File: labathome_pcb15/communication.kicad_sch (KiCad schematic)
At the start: 19 parts, among them M1 W5500_mini, SW2 ON RS TERM, SW3 ON CAN TERM, U1 MAX3485, U15 NRF24L01, U6 RFM95W-868S2, U7 SN65HVD230, X3 SIM7080G

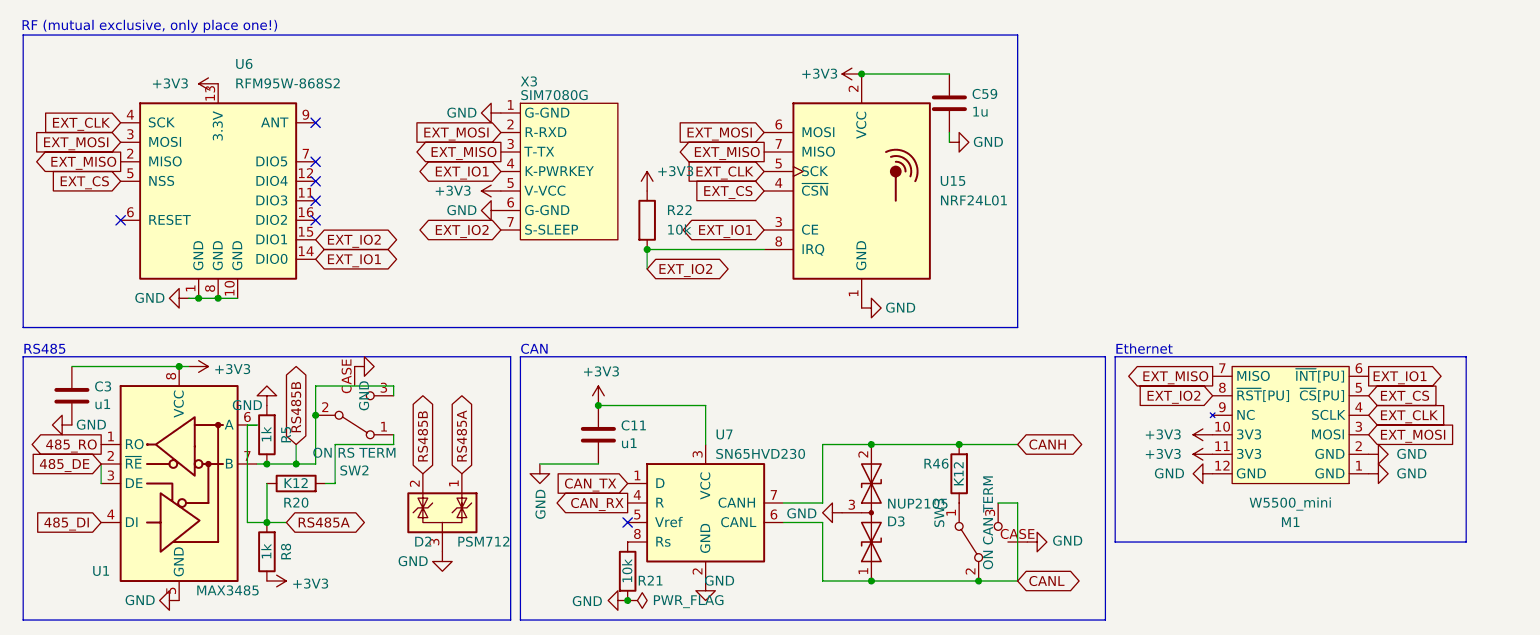
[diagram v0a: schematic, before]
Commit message: Minimal changes
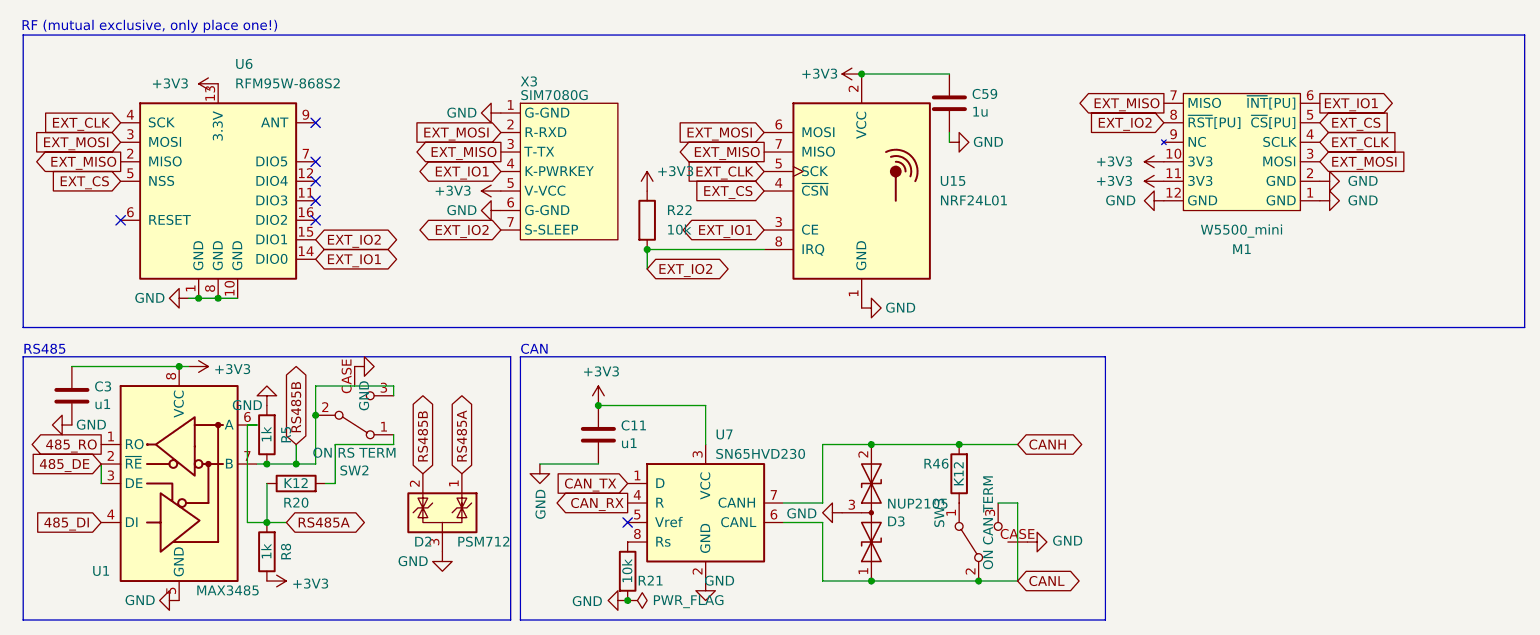
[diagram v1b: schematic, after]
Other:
- note removed: "Ethernet"
- moved on the sheet: M1
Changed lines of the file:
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@@
 		)
 	)
-	(polyline
-		(pts
-			(xy 156.21 58.42) (xy 156.21 82.55)
-		)
-		(stroke
-			(width 0)
-			(type default)
-		)
-	)
 	(wire
 		(pts
@@
 		)
 	)
-	(polyline
-		(pts
-			(xy 156.21 58.42) (xy 201.93 58.42)
-		)
-		(stroke
-			(width 0)
-			(type default)
-		)
-	)
 	(wire
 		(pts
@@
 		)
 	)
-	(polyline
-		(pts
-			(xy 201.93 82.55) (xy 156.21 82.55)
-		)
-		(stroke
-			(width 0)
-			(type default)
-		)
-	)
 	(wire
 		(pts
@@
 		)
 	)
-	(polyline
-		(pts
-			(xy 201.93 58.42) (xy 201.93 82.55)
-		)
-		(stroke
-			(width 0)
-			(type default)
-		)
-	)
 	(wire
 		(pts
@@
 	(rectangle
 		(start 13.97 16.51)
-		(end 143.51 54.61)
+		(end 209.55 54.61)
 		(stroke
 			(width 0)
@@
 		)
 	)
-	(text "Ethernet\n"
-		(exclude_from_sim no)
-		(at 156.21 58.42 0)
-		(effects
-			(font
-				(size 1.27 1.27)
-			)
-			(justify left bottom)
-		)
-	)
 	(text "CAN"
 		(exclude_from_sim no)
@@
 	(global_label "EXT_MISO"
 		(shape output)
-		(at 168.91 60.96 180)
+		(at 162.56 25.4 180)
 		(fields_autoplaced yes)
 		(effects
@@
 		)
 		(property "Intersheetrefs" "${INTERSHEET_REFS}"
-			(at 157.0349 60.96 0)
+			(at 150.6849 25.4 0)
 			(effects
 				(font
@@
 	(global_label "EXT_IO1"
 		(shape output)
-		(at 189.23 60.96 0)
+		(at 182.88 25.4 0)
 		(fields_autoplaced yes)
 		(effects
@@
 		)
 		(property "Intersheetrefs" "${INTERSHEET_REFS}"
-			(at 199.6537 60.96 0)
+			(at 193.3037 25.4 0)
 			(effects
 				(font
@@
 	(global_label "EXT_CS"
 		(shape input)
-		(at 189.23 63.5 0)
+		(at 182.88 27.94 0)
 		(fields_autoplaced yes)
 		(effects
@@
 		)
 		(property "Intersheetrefs" "${INTERSHEET_REFS}"
-			(at 198.9884 63.5 0)
+			(at 192.6384 27.94 0)
 			(effects
 				(font
@@
 	(global_label "EXT_MOSI"
 		(shape input)
-		(at 189.23 68.58 0)
+		(at 182.88 33.02 0)
 		(fields_autoplaced yes)
 		(effects
@@
 		)
 		(property "Intersheetrefs" "${INTERSHEET_REFS}"
-			(at 201.1051 68.58 0)
+			(at 194.7551 33.02 0)
 			(effects
 				(font
@@
 	(global_label "EXT_CLK"
 		(shape input)
-		(at 189.23 66.04 0)
+		(at 182.88 30.48 0)
 		(fields_autoplaced yes)
 		(effects
@@
 		)
 		(property "Intersheetrefs" "${INTERSHEET_REFS}"
-			(at 200.077 66.04 0)
+			(at 193.727 30.48 0)
 			(effects
 				(font
@@
 	(global_label "EXT_IO2"
 		(shape input)
-		(at 168.91 63.5 180)
+		(at 162.56 27.94 180)
 		(fields_autoplaced yes)
 		(effects
@@
 		)
 		(property "Intersheetrefs" "${INTERSHEET_REFS}"
-			(at 158.4863 63.5 0)
+			(at 152.1363 27.94 0)
 			(effects
 				(font
@@
 	(symbol
 		(lib_id "power:+3V3")
-		(at 168.91 68.58 90)
+		(at 162.56 33.02 90)
 		(unit 1)
 		(exclude_from_sim no)
@@
 		(dnp no)
 		(property "Reference" "#PWR0157"
-			(at 172.72 68.58 0)
+			(at 166.37 33.02 0)
 			(effects
 				(font
@@
 		)
 		(property "Value" "+3V3"
-			(at 160.02 68.58 90)
+			(at 153.67 33.02 90)
 			(effects
 				(font
@@
 		)
 		(property "Footprint" ""
-			(at 168.91 68.58 0)
+			(at 162.56 33.02 0)
 			(effects
 				(font
@@
 		)
 		(property "Datasheet" ""
-			(at 168.91 68.58 0)
+			(at 162.56 33.02 0)
 			(effects
 				(font
@@
 		)
 		(property "Description" "Power symbol creates a global label with name \"+3V3\""
-			(at 168.91 68.58 0)
+			(at 162.56 33.02 0)
 			(effects
 				(font
@@
 	(symbol
 		(lib_id "power:+3V3")
-		(at 168.91 71.12 90)
+		(at 162.56 35.56 90)
 		(unit 1)
 		(exclude_from_sim no)
@@
 		(dnp no)
 		(property "Reference" "#PWR0158"
-			(at 172.72 71.12 0)
+			(at 166.37 35.56 0)
 			(effects
 				(font
@@
 		)
 		(property "Value" "+3V3"
-			(at 160.02 71.12 90)
+			(at 153.67 35.56 90)
 			(effects
 				(font
@@
 		)
 		(property "Footprint" ""
-			(at 168.91 71.12 0)
+			(at 162.56 35.56 0)
 			(effects
 				(font
@@
 		)
 		(property "Datasheet" ""
-			(at 168.91 71.12 0)
+			(at 162.56 35.56 0)
 			(effects
 				(font
@@
 		)
 		(property "Description" "Power symbol creates a global label with name \"+3V3\""
-			(at 168.91 71.12 0)
+			(at 162.56 35.56 0)
 			(effects
 				(font
@@
 	(symbol
 		(lib_id "power:GND")
-		(at 189.23 73.66 90)
+		(at 182.88 38.1 90)
 		(unit 1)
 		(exclude_from_sim no)
@@
 		(dnp no)
 		(property "Reference" "#PWR0195"
-			(at 195.58 73.66 0)
+			(at 189.23 38.1 0)
 			(effects
 				(font
@@
 		)
 		(property "Value" "GND"
-			(at 196.85 73.66 90)
+			(at 190.5 38.1 90)
 			(effects
 				(font
@@
 		)
 		(property "Footprint" ""
-			(at 189.23 73.66 0)
+			(at 182.88 38.1 0)
 			(effects
 				(font
@@
 		)
 		(property "Datasheet" ""
-			(at 189.23 73.66 0)
+			(at 182.88 38.1 0)
 			(effects
 				(font
@@
 		)
 		(property "Description" "Power symbol creates a global label with name \"GND\" , ground"
-			(at 189.23 73.66 0)
+			(at 182.88 38.1 0)
 			(effects
 				(font
@@
 	(symbol
 		(lib_id "power:GND")
-		(at 189.23 71.12 90)
+		(at 182.88 35.56 90)
 		(unit 1)
 		(exclude_from_sim no)
@@
 		(dnp no)
 		(property "Reference" "#PWR0162"
-			(at 195.58 71.12 0)
+			(at 189.23 35.56 0)
 			(effects
 				(font
@@
 		)
 		(property "Value" "GND"
-			(at 196.85 71.12 90)
+			(at 190.5 35.56 90)
 			(effects
 				(font
@@
 		)
 		(property "Footprint" ""
-			(at 189.23 71.12 0)
+			(at 182.88 35.56 0)
 			(effects
 				(font
@@
 		)
 		(property "Datasheet" ""
-			(at 189.23 71.12 0)
+			(at 182.88 35.56 0)
 			(effects
 				(font
@@
 		)
 		(property "Description" "Power symbol creates a global label with name \"GND\" , ground"
-			(at 189.23 71.12 0)
+			(at 182.88 35.56 0)
 			(effects
 				(font
@@
 	(symbol
 		(lib_id "liebler_MODULES:W5500_mini")
-		(at 179.07 67.31 180)
+		(at 172.72 31.75 180)
 		(unit 1)
 		(exclude_from_sim no)
@@
 		(fields_autoplaced yes)
 		(property "Reference" "M1"
-			(at 179.07 80.01 0)
+			(at 172.72 44.45 0)
 			(effects
 				(font
@@
 		)
 		(property "Value" "W5500_mini"
-			(at 179.07 77.47 0)
+			(at 172.72 41.91 0)
 			(effects
 				(font
@@
 		)
 		(property "Footprint" "liebler_MODULES:W5500-mini"
-			(at 179.07 67.31 0)
+			(at 172.72 31.75 0)
 			(effects
 				(font
@@
 		)
 		(property "Datasheet" ""
-			(at 179.07 67.31 0)
+			(at 172.72 31.75 0)
 			(effects
 				(font
@@
 		)
 		(property "Description" ""
-			(at 179.07 67.31 0)
+			(at 172.72 31.75 0)
 			(effects
 				(font
@@
 	(symbol
 		(lib_id "power:GND")
-		(at 168.91 73.66 270)
+		(at 162.56 38.1 270)
 		(unit 1)
 		(exclude_from_sim no)
@@
 		(dnp no)
 		(property "Reference" "#PWR0161"
-			(at 162.56 73.66 0)
+			(at 156.21 38.1 0)
 			(effects
 				(font
@@
 		)
 		(property "Value" "GND"
-			(at 161.29 73.66 90)
+			(at 154.94 38.1 90)
 			(effects
 				(font
@@
 		)
 		(property "Footprint" ""
-			(at 168.91 73.66 0)
+			(at 162.56 38.1 0)
 			(effects
 				(font
@@
 		)
 		(property "Datasheet" ""
-			(at 168.91 73.66 0)
+			(at 162.56 38.1 0)
 			(effects
 				(font
@@
 		)
 		(property "Description" "Power symbol creates a global label with name \"GND\" , ground"
-			(at 168.91 73.66 0)
+			(at 162.56 38.1 0)
 			(effects
 				(font
